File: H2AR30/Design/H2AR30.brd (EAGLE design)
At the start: 34.6 x 30 mm, 59 parts, among them P1 HEXABIT_17.32, U2 INA199A2DCKT, U3 INA199A2DCKT, U4 TEXAS_INSTRUMENTS_REF3212AIDB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, X1 XTALL_CSTCE8M00G52

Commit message: some bugs fixed
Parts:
- U2, U3: value INA199A2DCKT -> INA199B2DCKT
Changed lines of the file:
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@@
 <attribute name="VALUE" x="6.26" y="-27.758" size="1.016" layer="27"/>
 </element>
-<element name="U2" library="HEXABITZ_ICs" library_urn="urn:adsk.eagle:library:20064554" package="SOT65P210X110-6N" package3d_urn="urn:adsk.eagle:package:19904117/2" value="INA199A2DCKT" x="9.906" y="-32.512" smashed="yes">
+<element name="U2" library="HEXABITZ_ICs" library_urn="urn:adsk.eagle:library:20064554" package="SOT65P210X110-6N" package3d_urn="urn:adsk.eagle:package:19904117/2" value="INA199B2DCKT" x="9.906" y="-32.512" smashed="yes">
 <attribute name="DESCRIPTION" value="26V, bi-directional current sense amplifier 6-SC70 -40 to 125" x="9.906" y="-32.512" size="1.778" layer="27" display="off"/>
 <attribute name="MFN" value="Texas Instruments" x="9.906" y="-32.512" size="1.778" layer="27" display="off"/>
-<attribute name="MPN" value="INA199A2DCKT" x="9.906" y="-32.512" size="1.778" layer="27" display="off"/>
+<attribute name="MPN" value="INA199B2DCKT" x="9.906" y="-32.512" size="1.778" layer="27" display="off"/>
 <attribute name="NAME" x="6.4516" y="-29.972" size="2.0828" layer="25" ratio="10" rot="SR0"/>
-<attribute name="OCTOPART_URL" value="https://octopart.com/ina199a2dckt-texas+instruments-18607270?r=sp" x="9.906" y="-32.512" size="1.778" layer="27" display="off"/>
+<attribute name="OCTOPART_URL" value="https://octopart.com/ina199b2dckt-texas+instruments-24258237?r=sp" x="9.906" y="-32.512" size="1.778" layer="27" display="off"/>
 <attribute name="VALUE" x="6.4516" y="-36.957" size="2.0828" layer="27" ratio="10" rot="SR0"/>
 </element>
@@
 <attribute name="VALUE" x="6.985" y="-108.839" size="1.27" layer="27"/>
 </element>
-<element name="U3" library="HEXABITZ_ICs" library_urn="urn:adsk.eagle:library:20064554" package="SOT65P210X110-6N" package3d_urn="urn:adsk.eagle:package:19904117/2" value="INA199A2DCKT" x="9.906" y="-112.903" smashed="yes">
+<element name="U3" library="HEXABITZ_ICs" library_urn="urn:adsk.eagle:library:20064554" package="SOT65P210X110-6N" package3d_urn="urn:adsk.eagle:package:19904117/2" value="INA199B2DCKT" x="9.906" y="-112.903" smashed="yes">
 <attribute name="DESCRIPTION" value="26V, bi-directional current sense amplifier 6-SC70 -40 to 125" x="9.906" y="-112.903" size="1.778" layer="27" display="off"/>
 <attribute name="MFN" value="Texas Instruments" x="9.906" y="-112.903" size="1.778" layer="27" display="off"/>
-<attribute name="MPN" value="INA199A2DCKT" x="9.906" y="-112.903" size="1.778" layer="27" display="off"/>
+<attribute name="MPN" value="INA199B2DCKT" x="9.906" y="-112.903" size="1.778" layer="27" display="off"/>
 <attribute name="NAME" x="6.4516" y="-110.363" size="2.0828" layer="25" ratio="10" rot="SR0"/>
-<attribute name="OCTOPART_URL" value="https://octopart.com/ina199a2dckt-texas+instruments-18607270?r=sp" x="9.906" y="-112.903" size="1.778" layer="27" display="off"/>
+<attribute name="OCTOPART_URL" value="https://octopart.com/ina199b2dckt-texas+instruments-24258237?r=sp" x="9.906" y="-112.903" size="1.778" layer="27" display="off"/>
 <attribute name="VALUE" x="6.4516" y="-117.348" size="2.0828" layer="27" ratio="10" rot="SR0"/>
 </element>

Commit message: some fixes
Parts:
- R10, R9: value 330k -> 1M
- R8: value 330K -> 1M
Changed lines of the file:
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@@
 <attribute name="VALUE" x="6.731" y="-94.234" size="1.27" layer="27"/>
 </element>
-<element name="R8" library="HEXABITZ_RCLS" library_urn="urn:adsk.eagle:library:20064561" package="R1206" package3d_urn="urn:adsk.eagle:package:23540/2" value="330K" x="8.255" y="-97.917" smashed="yes">
+<element name="R8" library="HEXABITZ_RCLS" library_urn="urn:adsk.eagle:library:20064561" package="R1206" package3d_urn="urn:adsk.eagle:package:23540/2" value="1M" x="8.255" y="-97.917" smashed="yes">
 <attribute name="NAME" x="6.985" y="-96.647" size="1.27" layer="25"/>
 <attribute name="POPULARITY" value="19" x="8.255" y="-97.917" size="1.778" layer="27" display="off"/>
@@
 <attribute name="VALUE" x="6.985" y="-100.457" size="1.27" layer="27"/>
 </element>
-<element name="R9" library="HEXABITZ_RCLS" library_urn="urn:adsk.eagle:library:20064561" package="R1206" package3d_urn="urn:adsk.eagle:package:23540/2" value="330k" x="8.255" y="-102.108" smashed="yes">
+<element name="R9" library="HEXABITZ_RCLS" library_urn="urn:adsk.eagle:library:20064561" package="R1206" package3d_urn="urn:adsk.eagle:package:23540/2" value="1M" x="8.255" y="-102.108" smashed="yes">
 <attribute name="NAME" x="6.985" y="-100.838" size="1.27" layer="25"/>
 <attribute name="POPULARITY" value="19" x="8.255" y="-102.108" size="1.778" layer="27" display="off"/>
@@
 <attribute name="VALUE" x="6.985" y="-104.648" size="1.27" layer="27"/>
 </element>
-<element name="R10" library="HEXABITZ_RCLS" library_urn="urn:adsk.eagle:library:20064561" package="R1206" package3d_urn="urn:adsk.eagle:package:23540/2" value="330k" x="8.255" y="-106.299" smashed="yes">
+<element name="R10" library="HEXABITZ_RCLS" library_urn="urn:adsk.eagle:library:20064561" package="R1206" package3d_urn="urn:adsk.eagle:package:23540/2" value="1M" x="8.255" y="-106.299" smashed="yes">
 <attribute name="NAME" x="6.985" y="-105.029" size="1.27" layer="25"/>
 <attribute name="POPULARITY" value="19" x="8.255" y="-106.299" size="1.778" layer="27" display="off"/>

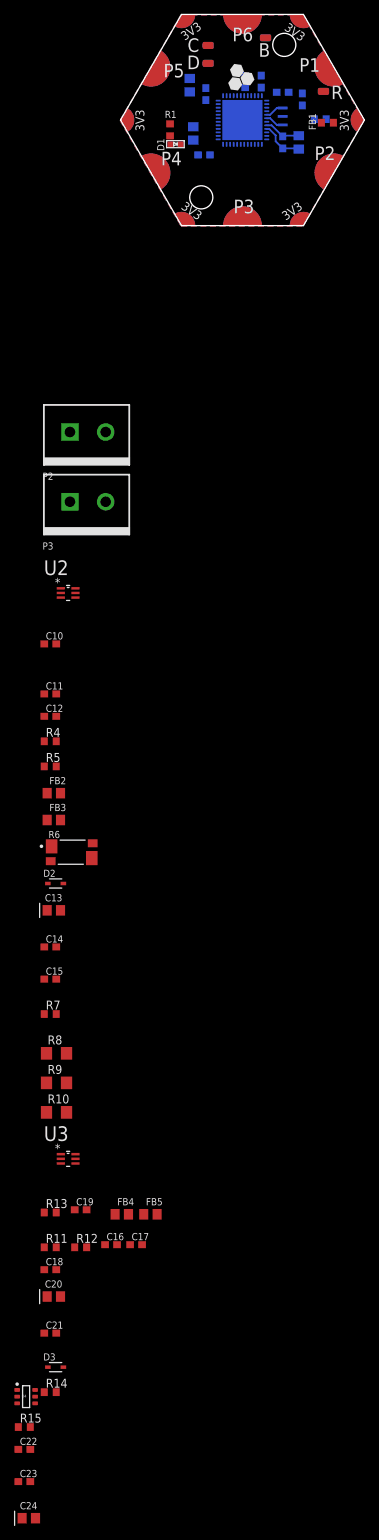
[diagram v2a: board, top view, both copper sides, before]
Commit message: no message
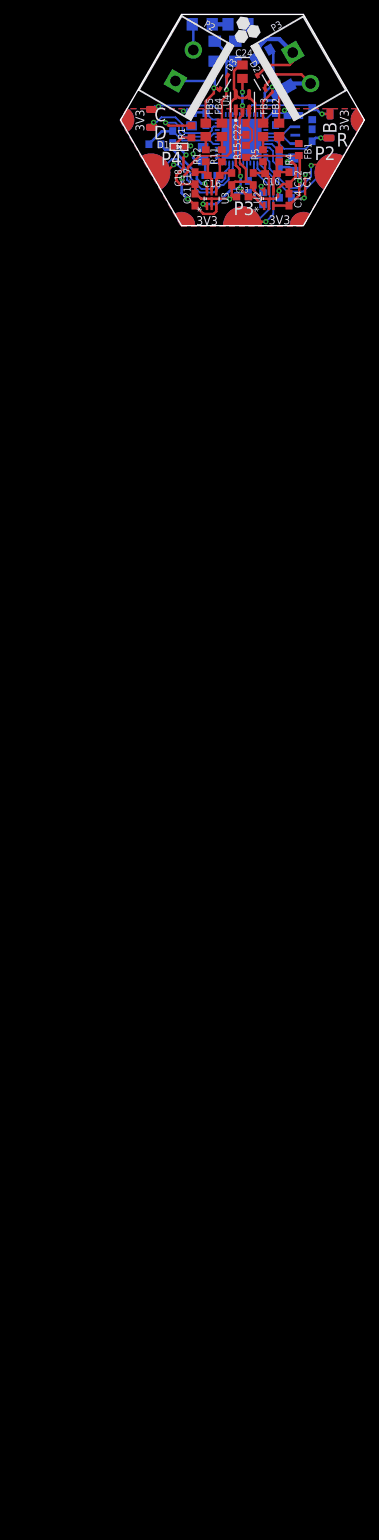
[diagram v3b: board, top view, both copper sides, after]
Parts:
- removed C13, C20: 1.00uF, HEXABITZ_RCLS:C-0805-POL
- P1: value HEXABIT_17.32 -> HEXABIT__NO_P1_P5_P6_P7_P12; device hexabitz_connectors:HEXABIT_17.32 -> hexabitz_connectors:HEXABIT_17.32_NO_P1_P6_P5_P7_P12
- R10, R8, R9: value 1M -> 1M0
- R11, R12, R4, R5: value 1.01R -> 1R0
- R14: value 3.3K -> 150R; device HEXABITZ_RCLS:R-0603 -> HEXABITZ_RCLS:R1206
- U3: value INA199B2DCKT -> INA199B1DCKT
- U4: value TEXAS_INSTRUMENTS_REF3212AIDBVRTEXAS_INSTRUMENTS_REF3212AIDBVR_0_0 -> TEXAS_INSTRUMENTS_REF2033AIDDCRTEXAS_INSTRUMENTS_REF2033AIDDCR_0_2; device HEXABITZ_ICs:TEXAS_INSTRUMENTS_REF3212AIDBVR_0 -> HEXABITZ_ICs:TEXAS_INSTRUMENTS_REF2033AIDDCR_2
- moved C24 207.7 mm to (34.7, 41.5), turned to 270 degrees
- moved R14 191.9 mm to (30.7, 44.5), flipped to the bottom, turned to 90 degrees
- moved C22 190.2 mm to (35.2, 33.4), turned to 270 degrees
- moved U4 186.4 mm to (34.7, 37.2), turned to 90 degrees
- moved C23 185.1 mm to (34.7, 23.7), turned to 180 degrees
- moved D3 184.1 mm to (32.0, 40.0), turned to 60 degrees
- moved R15 183.9 mm to (35.2, 30.2), turned to 270 degrees
- moved C21 162.3 mm to (27.9, 23.4), turned to 90 degrees
- moved R11 157.0 mm to (31.8, 29.6), turned to 270 degrees
- moved C18 156.4 mm to (27.9, 26.4), turned to 270 degrees
- moved R12 156.1 mm to (29.5, 29.6), turned to 270 degrees
- moved FB4 154.7 mm to (31.8, 33.3), turned to 270 degrees
- moved FB5 154.3 mm to (29.5, 33.3), turned to 270 degrees
- moved C19 153.0 mm to (24.8, 32.3), flipped to the bottom, turned to 270 degrees
- moved R10 152.9 mm to (33.7, 44.5), flipped to the bottom, turned to 90 degrees
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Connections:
- net N$13 renamed CURRENT_P
- net N$14 renamed CURRENT_N
- removed net USART1_RX: P1.PAD_PD5, U1.P$31
- removed net USART1_TX: P1.PAD_PU5, U1.P$30
- removed net USART4_RX: P1.PAD_PD1, U1.P$11
- removed net USART4_TX: P1.PAD_PU1, U1.P$10
- removed net VDDA: C1.1, C13.1, C14.1, C2.1, C20.1, C21.1, C24.1, FB1.1, U1.P$9
- removed net VSSA: C1.2, C13.2, C14.2, C2.2, C20.2, C21.2, C24.2, R2.2, U1.P$8
- net AGND: now also C1.2, C14.2, C2.2, C21.2, C24.2, R2.2, U1.P$8; no longer U4.1
- net CURRENT_SENSE: now also U1.P$17; no longer U1.P$29
- net GND: now also U1.P$2, U1.P$20, U1.P$27, U1.P$28, U1.P$3; no longer P1.PAD_PD12, P1.PAD_PD7
- net NEUTRAL: now also P2.1; no longer P2.2
- net PHASE: now also P2.2; no longer P2.1
- net USART5_RX: no longer P1.PAD_PD6
- net USART5_TX: no longer P1.PAD_PU6
- net VCC: now also C1.1, C14.1, C2.1, C21.1, C24.1, FB1.1, U1.P$9, U4.5
- net VDD: no longer P1.PAD_PU12, P1.PAD_PU7
- net VOLTAGE_SENSE: now also U1.P$29; no longer U1.P$17
- net V_REF: now also U4.1; no longer U4.5, U4.6
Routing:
- net VCC: track 0.00 -> 68.7 mm, vias 0 -> 3
- net AGND: track 0.00 -> 64.8 mm, vias 0 -> 6
- net V_REF: track 0.00 -> 22.8 mm, vias 0 -> 3
- net VDD: track 0.00 -> 18.0 mm, vias 0 -> 3
- net N$21: track 0.00 -> 16.7 mm, vias 0 -> 1
- net USART3_TX: track 0.00 -> 16.2 mm, vias 0 -> 1
- net NEUTRAL: track 0.00 -> 15.8 mm, vias 0 -> 1
- net USART3_RX: track 0.00 -> 15.8 mm
- net CT_1: track 0.00 -> 14.9 mm
- net B1: track 0.00 -> 14.4 mm, vias 0 -> 1
- net USART2_TX: track 0.00 -> 14.0 mm, vias 0 -> 1
- net USART6_TX: track 0.00 -> 13.1 mm, vias 0 -> 1
- net N$7: track 0.00 -> 13.0 mm, vias 0 -> 1
- net USART2_RX: track 0.00 -> 12.9 mm
- net N$3: track 0.00 -> 12.7 mm, vias 0 -> 1
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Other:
- board text added: "CT1"
- board text added: "CT2"
- board text added: "N"
- board text added: "PH"
- board text removed: "P1"
- board text removed: "P5"
- board text removed: "P6"

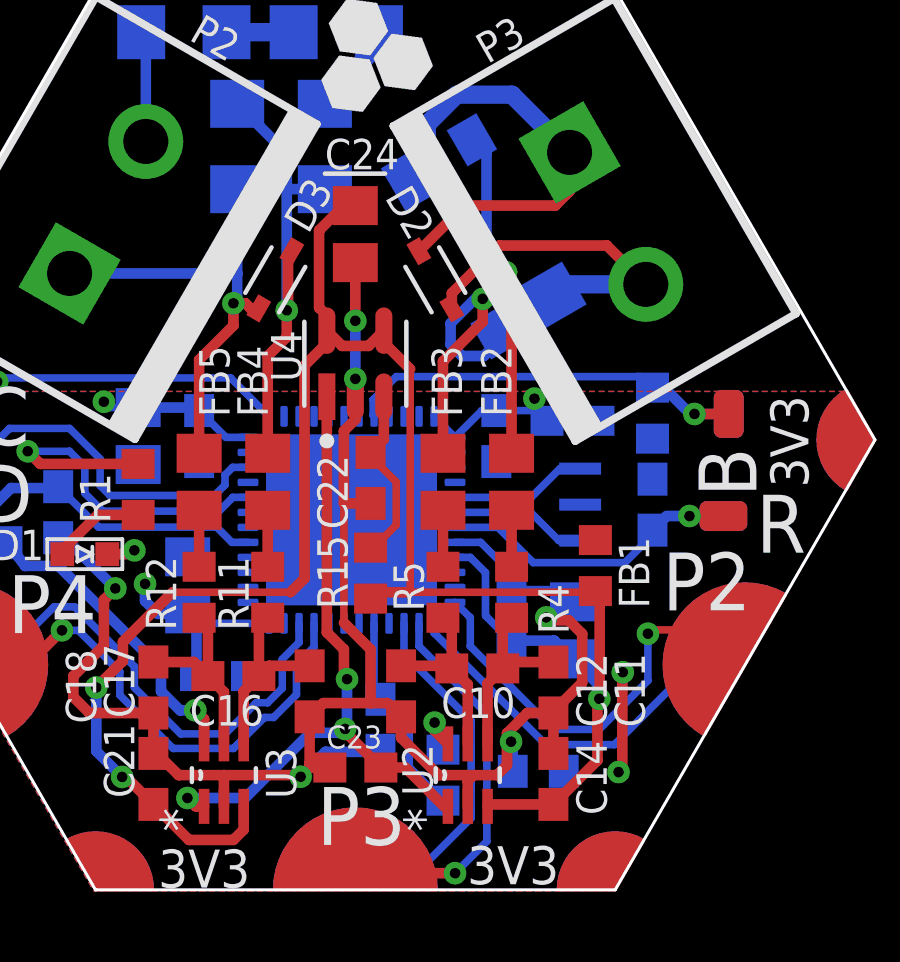
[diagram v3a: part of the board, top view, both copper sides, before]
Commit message: no message
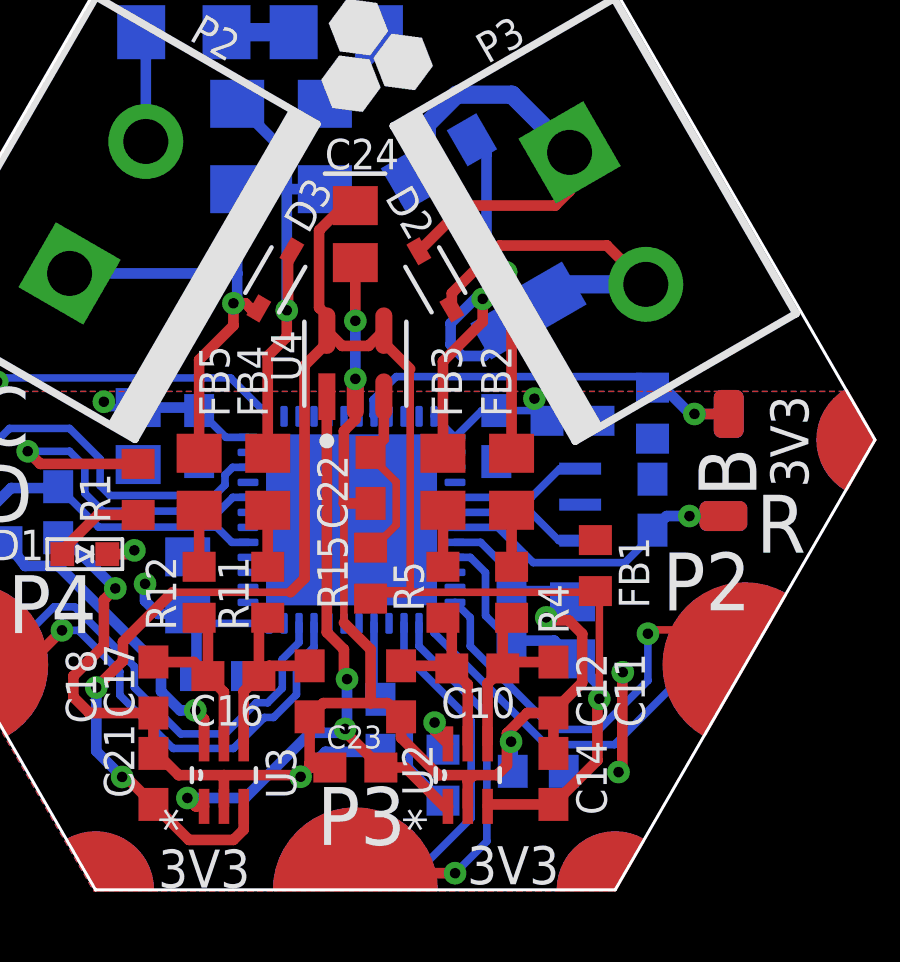
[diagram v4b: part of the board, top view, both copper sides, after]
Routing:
- net N$21: track 16.7 -> 15.9 mm
